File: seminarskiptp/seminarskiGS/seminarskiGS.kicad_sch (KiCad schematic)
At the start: 12 parts, among them J1 Screw_Terminal_01x02, J2 Conn_01x04_Pin, SW1 SW_Push, U1 AT89C4051-24P, U2 LCD-016N002L, Y1 11.0592MHz

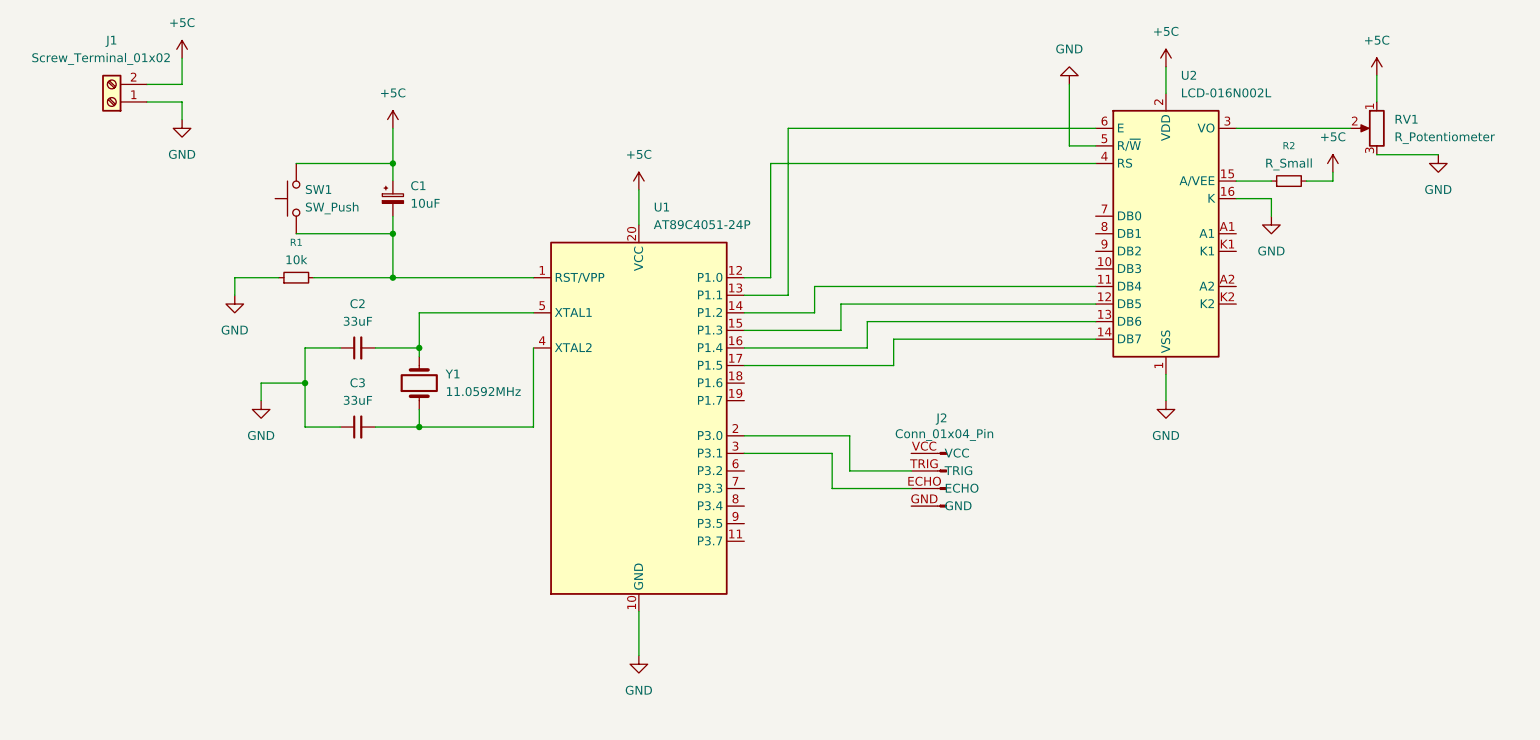
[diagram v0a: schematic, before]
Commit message: 26.1.
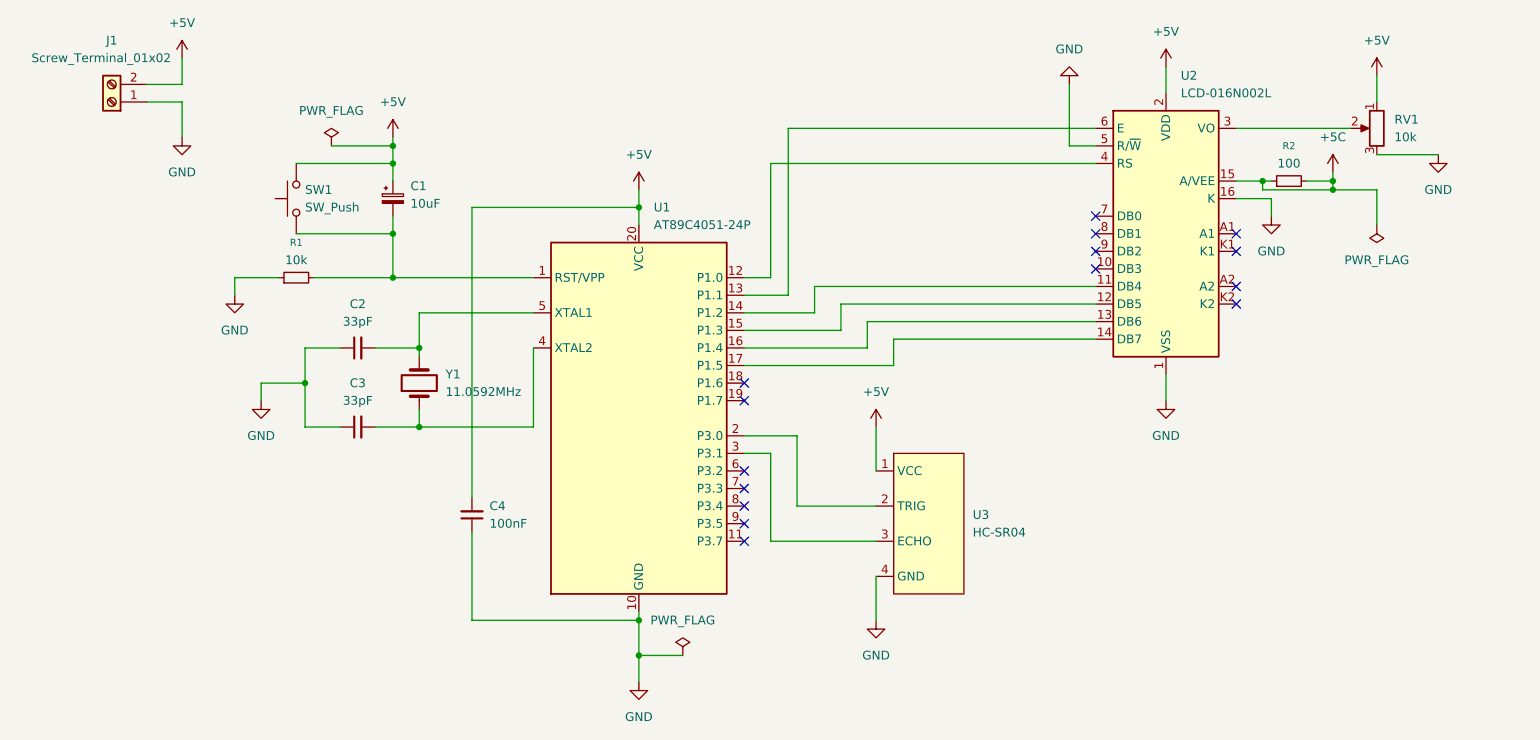
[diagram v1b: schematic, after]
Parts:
- removed J2: Conn_01x04_Pin, symbol Connector:Conn_01x04_Pin
- added C4: 100nF, Capacitor_THT:C_Disc_D3.0mm_W2.0mm_P2.50mm, symbol Device:C_Small
- added U3: HC-SR04, Libraryfootprint:HC-SR04_, symbol custom symbol:HC-SR04_
- C1: footprint (none) -> Capacitor_THT:CP_Radial_Tantal_D5.0mm_P2.50mm
- C2, C3: value 33uF -> 33pF; footprint (none) -> Capacitor_THT:C_Disc_D3.0mm_W2.0mm_P2.50mm
- J1: footprint (none) -> TerminalBlock_Phoenix:TerminalBlock_Phoenix_MKDS-1,5-2-5.08_1x02_P5.08mm_Horizontal
- R1: footprint (none) -> Resistor_THT:R_Axial_DIN0207_L6.3mm_D2.5mm_P7.62mm_Horizontal
- R2: value R_Small -> 100; footprint (none) -> Resistor_THT:R_Axial_DIN0207_L6.3mm_D2.5mm_P7.62mm_Horizontal
- RV1: value R_Potentiometer -> 10k; footprint (none) -> Potentiometer_THT:Potentiometer_Bourns_3386W_Horizontal
- SW1: footprint (none) -> Button_Switch_THT:SW_PUSH_6mm
- Y1: footprint (none) -> Crystal:Crystal_HC49-U_Horizontal
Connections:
- net +5C: now also R2.1, U2.15 (A/VEE); no longer C1.1, J1.2 (Pin_2), RV1.1, SW1.2, U1.20 (VCC), U2.2 (VDD)
- net GND: now also C4.1, U3.4 (GND)
- net at U1.2 (P3.0): now also U3.2 (TRIG)
- net at U1.3 (P3.1): now also U3.3 (ECHO)
- new net +5V: C1.1, C4.2, J1.2 (Pin_2), RV1.1, SW1.2, U1.20 (VCC), U2.2 (VDD), U3.1 (VCC)
- no-connect marks 0 -> 15
